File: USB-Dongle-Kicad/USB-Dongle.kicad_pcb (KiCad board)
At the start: 2 copper layers, 33 x 40 mm, 19 parts, among them J1 USB_C_Receptacle_USB2.0_16P, J2 Conn_01x04_Pin, J3 Conn_01x06_Pin, J4 Conn_01x06_Pin, SW1 SW_SPDT_312, U1 CH340C, U2 TLV75533PDBVR

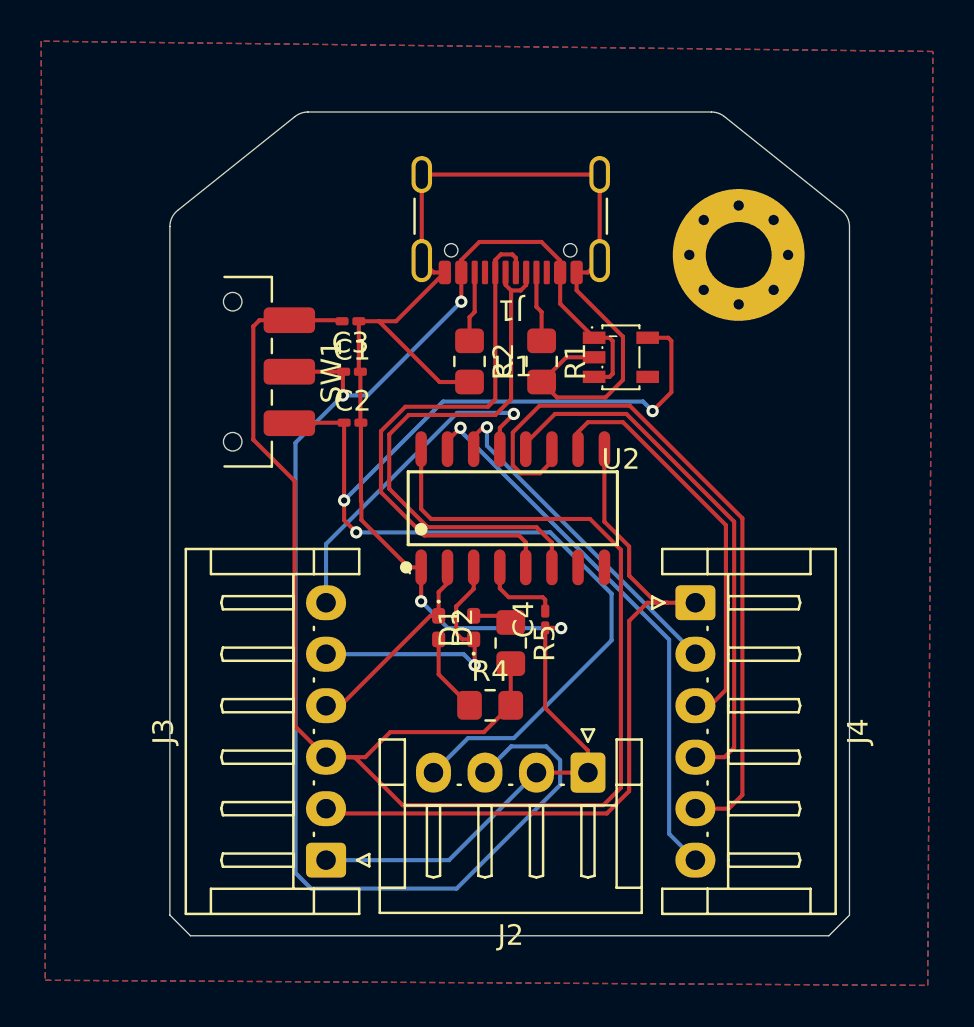
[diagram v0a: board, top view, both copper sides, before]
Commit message: Updated stuff
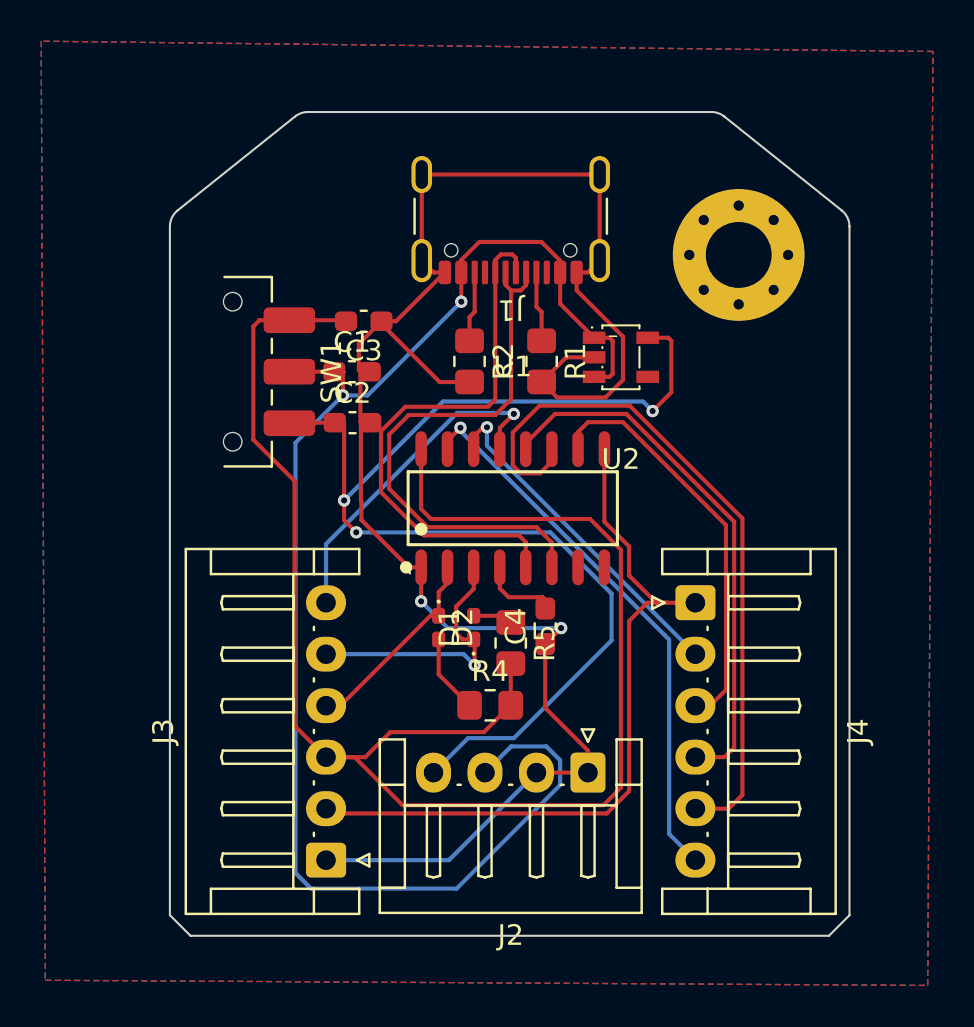
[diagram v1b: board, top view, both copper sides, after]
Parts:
- C1, C2, C3, C4: footprint Capacitor_SMD:C_0201_0603Metric_Pad0.64x0.40mm_HandSolder -> Capacitor_SMD:C_0603_1608Metric_Pad1.08x0.95mm_HandSolder
- moved C3 0.65 mm to (160.9, 40.0)
- moved C4 0.33 mm to (169.7, 54.9)
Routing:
- net GND: track 90.0 -> 89.1 mm
